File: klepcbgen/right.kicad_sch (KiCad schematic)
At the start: 80 parts, among them K10 ),0,,F10, K11 _,-,,F11, K12 +,=,,F12, K13 Backspace, K14 Delete,Insert, K21 Y, K22 U, K23 I, K24 O, K25 P, K26 {,[, K27 },], K28 |,\, K29 ~~,`, K36 H, K37 J, K38 K, K39 L, K40 :,;, K41 ",', K42 Enter, K43 Home,PgUp, K50 N, K51 M, K52 <,,, K53 >,., K54 ?,/, K55 Shift, K56 ↑, K57 End,PgDn, K62 Space, K63 Alt, K64 Fn, K65 Ctrl, K66 ←, K67 ↓, K68 →, K7 &,7,,F7, K8 *,8,,F8, K9 (,9,,F9

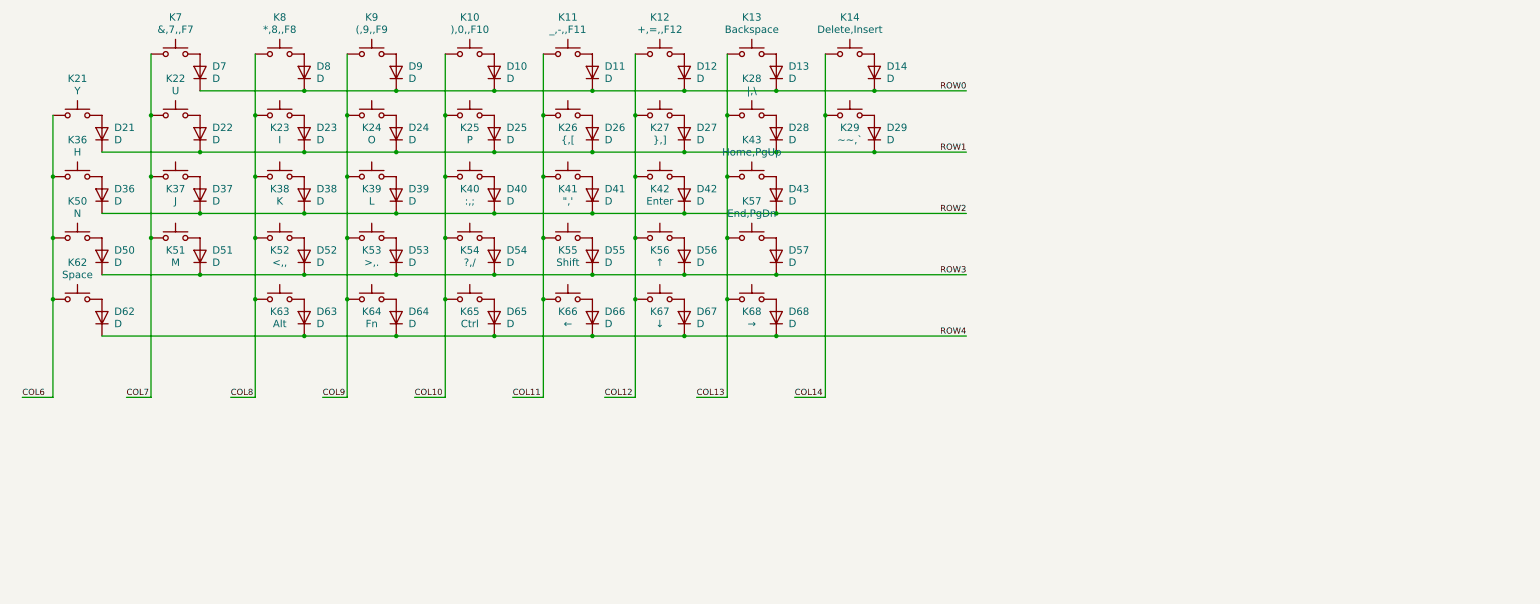
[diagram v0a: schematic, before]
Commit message: Moved things around more so that they make sense. Slowly figuring it out.
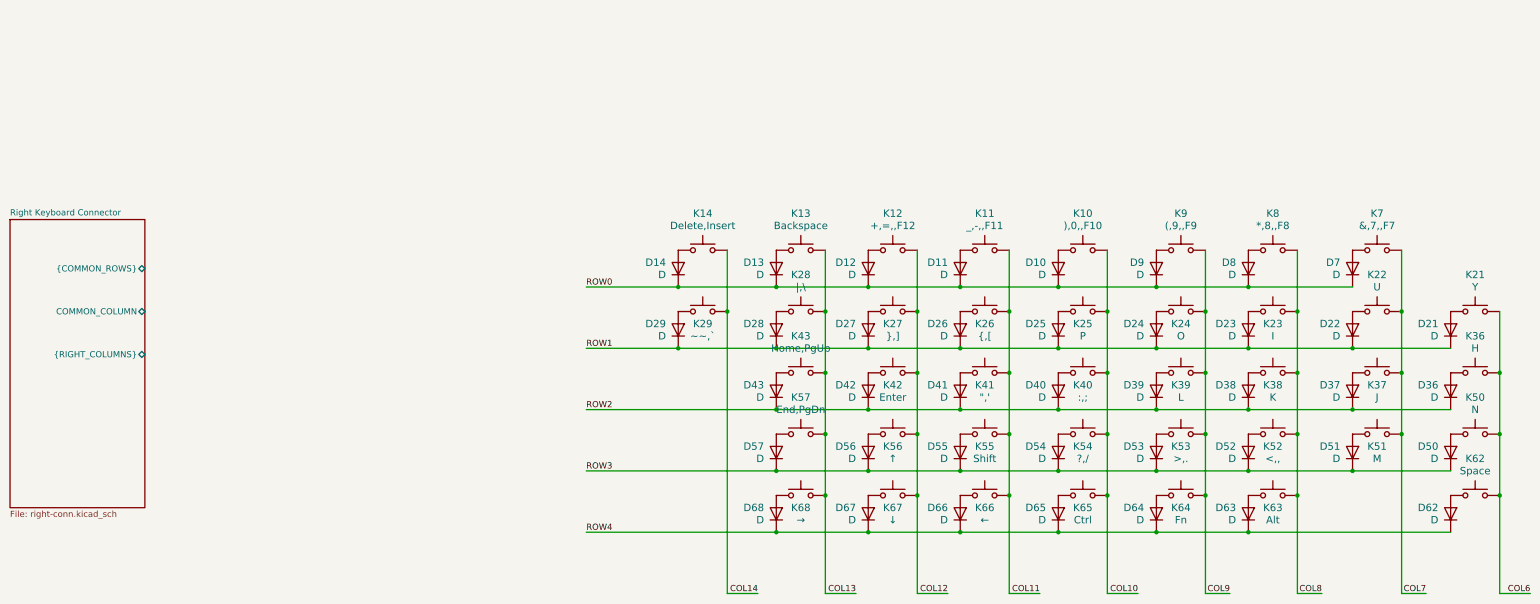
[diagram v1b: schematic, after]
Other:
- added sheet Right Keyboard Connector (right-conn.kicad_sch)
- moved on the sheet: D10, D11, D12, D13, D14, D21, D22, D23, D24, D25, D26, D27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
